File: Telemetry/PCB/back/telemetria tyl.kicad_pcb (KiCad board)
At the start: 2 copper layers, 60 parts, among them J1 Conn_01x26_Male, U1 STM32F405RGTx, U2 MCP2561-E-SN, Y1 Crystal_GND24_Small

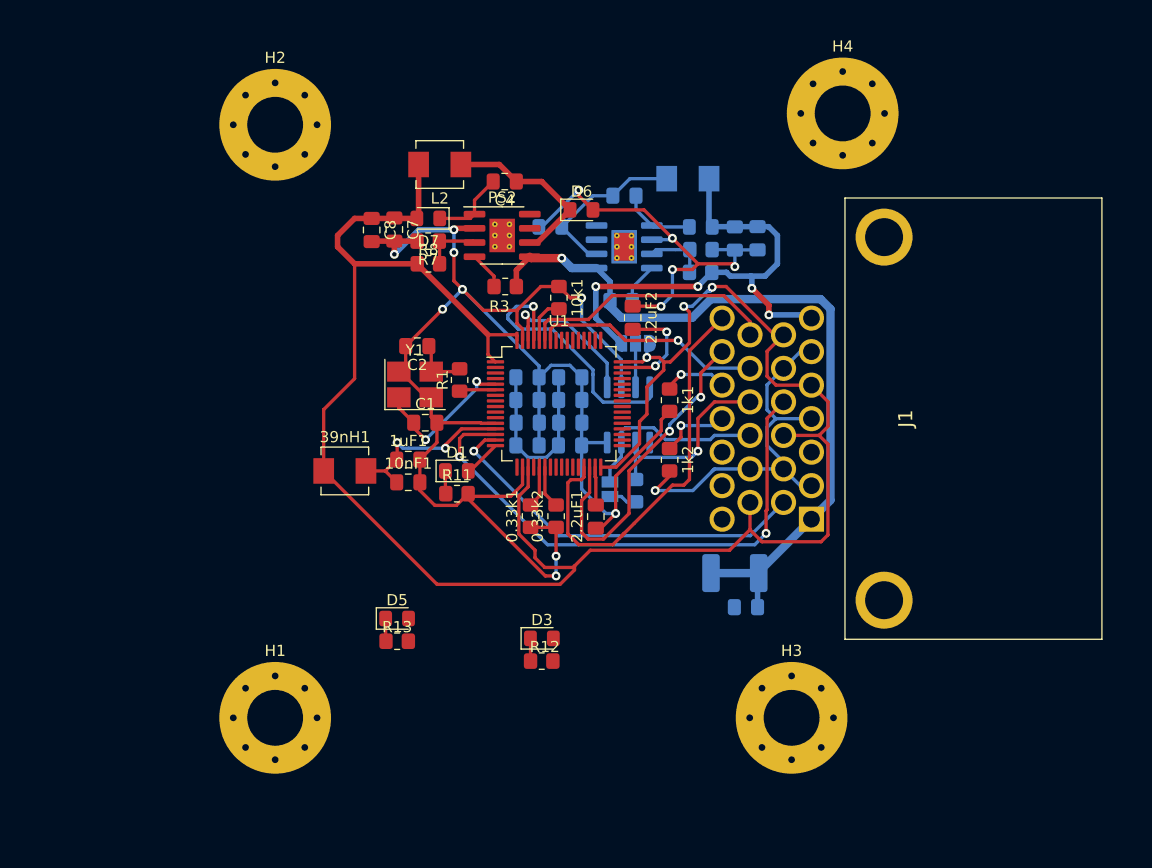
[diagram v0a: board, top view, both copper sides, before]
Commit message: Telemetry back v1.0 (#27)
* init commit

* New brd design & final scheme

* final scheme & 60%pcb

* almost finished - space for Bartek

* pre_finnal

* pre_finnal

* telemetry_back_finnal

* Telemetry_back_finnal

* kicad libs

* Create _autosave-telemetria tyl.sch

* Telemetry_back_finnal

* finnal

* Remove Dashboard files from this branch

This reverts commit ffcd00ee911598f18239aabaf1713ea3aea0f91a.

Co-authored-by: wojtekszamocki <w.szamocki.02@gmail.com>
Co-authored-by: Bartosz Janicki <janicki.bartosz.0@gmail.com>
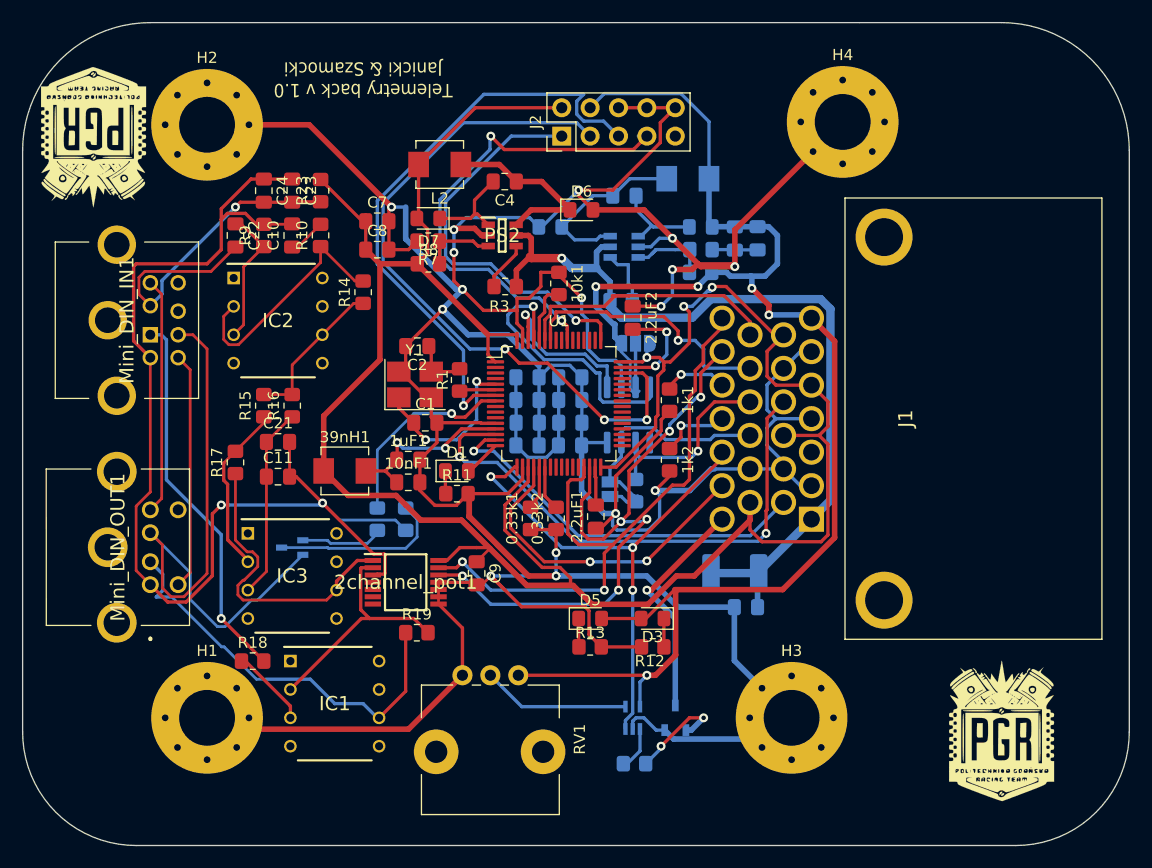
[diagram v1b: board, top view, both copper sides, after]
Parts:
- added 2channel_pot1: MAX5478EUD+T, SamacSys_Parts:SOP65P640X110-14N, F.Cu at (53.3, 66.6)
- added BJT1: BC846BW,115, SamacSys_Parts:SOT65P210X110-3N, B.Cu at (43.2, 63.5)
- added C10: C, Capacitor_SMD:C_0805_2012Metric_Pad1.18x1.45mm_HandSolder, F.Cu at (43.2, 35.6)
- added C11: C, Capacitor_SMD:C_0805_2012Metric_Pad1.18x1.45mm_HandSolder, F.Cu at (41.9, 57.1)
- added C21: C, Capacitor_SMD:C_0805_2012Metric_Pad1.18x1.45mm_HandSolder, F.Cu at (41.9, 54.0)
- added C22: C, Capacitor_SMD:C_0805_2012Metric_Pad1.18x1.45mm_HandSolder, F.Cu at (38.1, 35.6)
- added C23: ?, Capacitor_SMD:C_0805_2012Metric_Pad1.18x1.45mm_HandSolder, F.Cu at (43.2, 31.6)
- added C24: 10uF, Capacitor_SMD:C_0805_2012Metric_Pad1.18x1.45mm_HandSolder, F.Cu at (40.6, 31.6)
- added C9: 0.1uF, Capacitor_SMD:C_0805_2012Metric_Pad1.18x1.45mm_HandSolder, F.Cu at (59.7, 65.8)
- added G***: LOGO, SamacSys_Parts:logo, F.Cu at (106.7, 80.0)
- added G***: LOGO, SamacSys_Parts:logo, F.Cu at (25.4, 26.7)
- added IC1: LM741CN_NOPB, DIP794W53P254L959H508Q8N, F.Cu at (47.0, 77.5)
- added IC2: LM741CN_NOPB, DIP794W53P254L959H508Q8N, F.Cu at (41.9, 43.2)
- added IC3: LM741CN_NOPB, DIP794W53P254L959H508Q8N, F.Cu at (43.2, 66.0)
- added IC4: NCX2200GW,125, SamacSys_Parts:NCX2200GW, B.Cu at (73.7, 78.7)
- added J2: Conn_02x05_Odd_Even, Connector_PinHeader_2.54mm:PinHeader_2x05_P2.54mm_Vertical, F.Cu at (67.3, 26.7)
- added Mini_DIN_IN1: 5749268-1, SamacSys_Parts:57492681, F.Cu at (30.5, 44.5)
- added Mini_DIN_OUT1: 5750071-1, SamacSys_Parts:57500711, F.Cu at (30.5, 64.8)
- added Q1: PMV280ENEAR, SamacSys_Parts:PMV280ENEAR, B.Cu at (77.5, 78.7)
- added R10: R, Resistor_SMD:R_0805_2012Metric_Pad1.20x1.40mm_HandSolder, F.Cu at (45.7, 35.6)
- added R14: R, Resistor_SMD:R_0805_2012Metric_Pad1.20x1.40mm_HandSolder, F.Cu at (49.5, 40.6)
- added R15: R, Resistor_SMD:R_0805_2012Metric_Pad1.20x1.40mm_HandSolder, F.Cu at (40.6, 50.8)
- added R16: R, Resistor_SMD:R_0805_2012Metric_Pad1.20x1.40mm_HandSolder, F.Cu at (43.2, 50.8)
- added R17: R, Resistor_SMD:R_0805_2012Metric_Pad1.20x1.40mm_HandSolder, F.Cu at (38.1, 55.9)
- added R18: R, Resistor_SMD:R_0805_2012Metric_Pad1.20x1.40mm_HandSolder, F.Cu at (39.6, 73.7)
- added R19: R?, Resistor_SMD:R_0805_2012Metric_Pad1.20x1.40mm_HandSolder, F.Cu at (54.3, 71.1)
- added R20: 3.3k, Resistor_SMD:R_0805_2012Metric_Pad1.20x1.40mm_HandSolder, B.Cu at (73.8, 82.8)
- added R21: 4.7k, Resistor_SMD:R_0805_2012Metric_Pad1.20x1.40mm_HandSolder, B.Cu at (50.8, 61.0)
- added R22: 1k, Resistor_SMD:R_0805_2012Metric_Pad1.20x1.40mm_HandSolder, B.Cu at (53.3, 61.0)
- added R23: R, Resistor_SMD:R_0805_2012Metric_Pad1.20x1.40mm_HandSolder, F.Cu at (45.7, 31.6)
- added R9: 1M, Resistor_SMD:R_0805_2012Metric_Pad1.20x1.40mm_HandSolder, F.Cu at (40.6, 35.6)
- added RV1: R_POT, Potentiometer_THT:Potentiometer_Alps_RK09L_Single_Vertical, F.Cu at (58.4, 74.9)
- PS1, PS2: footprint Package_SO:SOIC-8-1EP_3.9x4.9mm_P1.27mm_EP2.29x3mm_ThermalVias -> SamacSys_Parts:SOT95P280X145-6N
- R4: value R -> 120
- moved D5 17.3 mm to (69.8, 69.8)
- moved R13 17.3 mm to (69.8, 72.4)
- moved D3 10.1 mm to (75.4, 69.8), turned to 180 degrees
- moved R12 10.0 mm to (75.5, 72.4), turned to 180 degrees
- moved H1 6.10 mm to (35.6, 78.7)
- moved H2 6.10 mm to (35.6, 25.7)
- moved C8 1.83 mm to (50.8, 36.8), turned to 0 degrees
- moved C7 1.69 mm to (50.8, 34.3), turned to 0 degrees
- moved 10k1 1.27 mm to (67.1, 39.9)
- moved H4 0.76 mm to (92.5, 25.4)
- moved 0.33k1 0.20 mm to (64.5, 60.9)
- moved 0.33k2 0.20 mm to (66.8, 60.9)
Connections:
- net ADC1_IN0 renamed ADC1_IN0_AMORKI
- net ADC2_IN1 renamed ADC2_IN1_AMORKI
- C13 pad 1: Net-(C13-Pad1) -> +3V3
- C14 pad 1: Net-(C13-Pad1) -> +3V3
- C15 pad 1: Net-(C13-Pad1) -> +3V3
- C16 pad 1: Net-(C13-Pad1) -> +3V3
- C17 pad 1: Net-(C13-Pad1) -> +3V3
- C18 pad 1: Net-(C13-Pad1) -> +3V3
- C19 pad 1: Net-(C13-Pad1) -> +3V3
- C20 pad 1: Net-(C13-Pad1) -> +3V3
- J1 pad 24: Net-(J1-Pad24) -> BREAK_PRESSURE_0
- J1 pad 25: Net-(J1-Pad25) -> BREAK_PRESSURE_ADC
- J1 pad 26: Net-(J1-Pad26) -> LED_GND
- R4 pad 1: Net-(JP2-Pad1) -> CAN_H1
- U1 pad 17: Net-(U1-Pad17) -> BREAK_PRESSURE_0
- U1 pad 20: Net-(U1-Pad20) -> BREAK_PRESSURE_ADC
- U1 pad 8: Net-(U1-Pad8) -> PTT
- U2 pad 3: Net-(JP1-Pad2) -> +5V
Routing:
- net GND: track 231.4 -> 445.9 mm, vias 15 -> 16
- net GND_MIC&ANC: track 0.00 -> 105.7 mm, vias 0 -> 2
- net +5V: track 48.7 -> 139.7 mm, vias 4 -> 5
- net +3V3: track 190.3 -> 268.3 mm
- net SWDIO: track 0.00 -> 62.9 mm, vias 0 -> 3
- net GND_SPK: track 0.00 -> 55.0 mm
- net NRST: track 0.00 -> 53.8 mm, vias 0 -> 1
- net BREAK_PRESSURE_0: track 0.00 -> 46.4 mm, vias 0 -> 3
- net SWO: track 0.00 -> 43.8 mm, vias 0 -> 2
- net V_OUT: track 0.00 -> 36.9 mm
- net SWCLK: track 0.00 -> 35.6 mm, vias 0 -> 1
- net V_MIC: track 0.00 -> 34.0 mm, vias 0 -> 1
- net V_ANC: track 0.00 -> 32.5 mm, vias 0 -> 1
- net BREAK_PRESSURE_ADC: track 0.00 -> 29.3 mm, vias 0 -> 2
- net 12C2_SDA: track 29.8 -> 57.3 mm, vias 2 -> 6
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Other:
- board outline added: 99.1 x 73.7 mm
- board text added: "Telemetry back v 1.0 Janicki & Szamocki"
- board text added: "Telemetry back v 1.0 Szamocki & Janicki"
